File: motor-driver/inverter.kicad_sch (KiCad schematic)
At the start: 37 parts

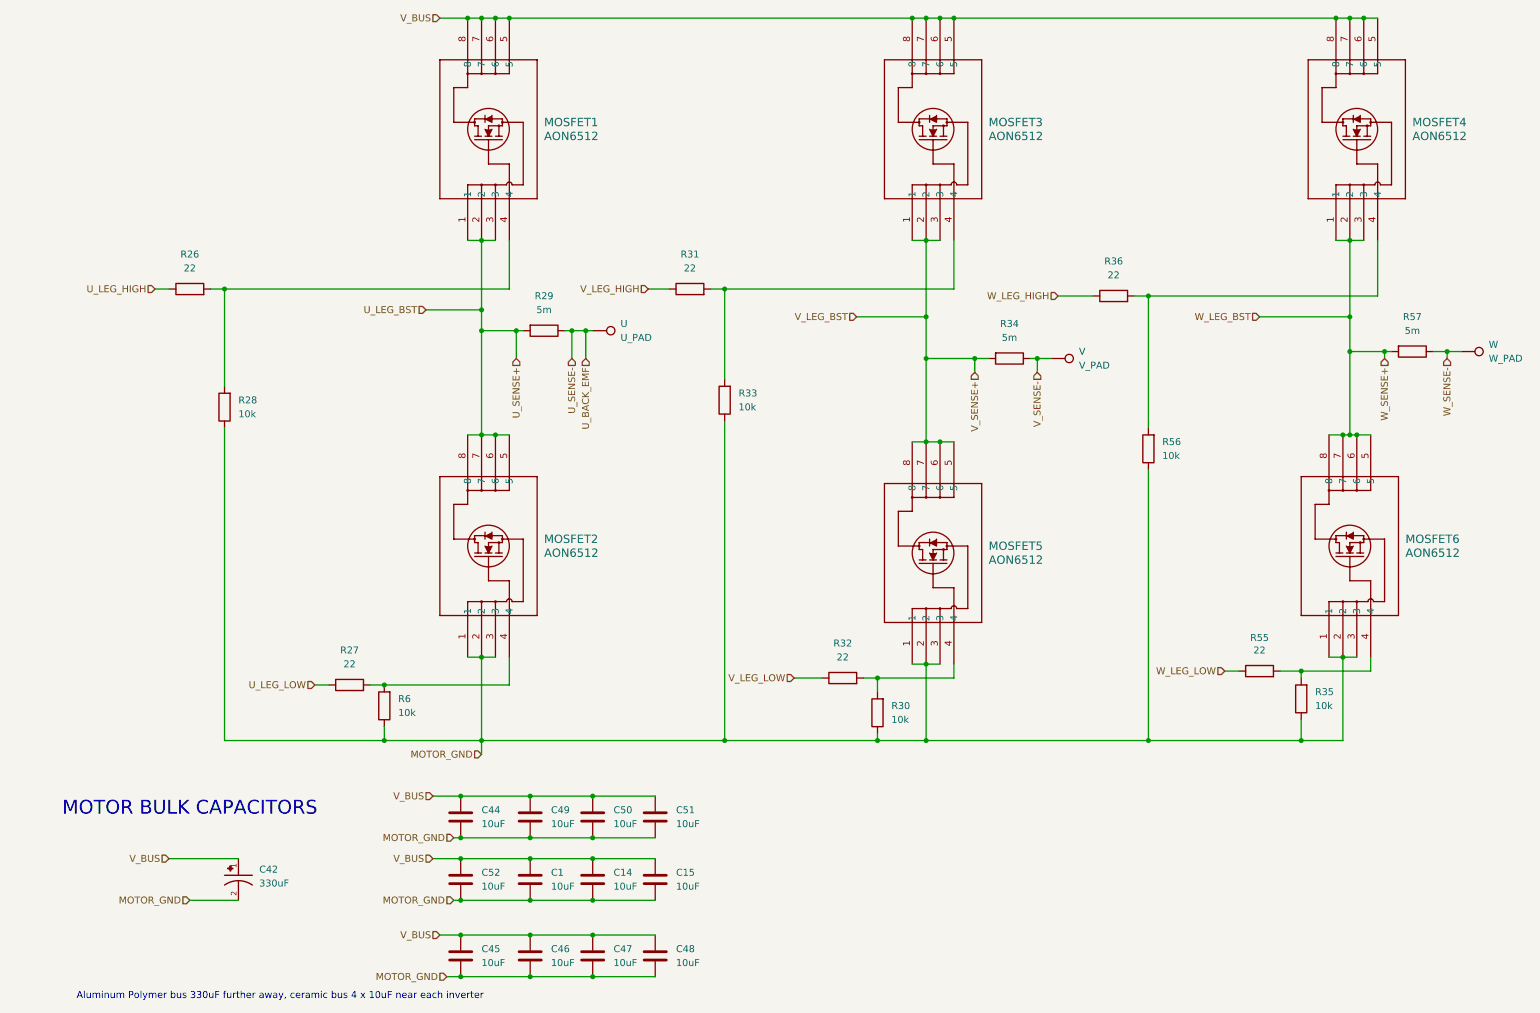
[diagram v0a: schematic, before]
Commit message: post revisions
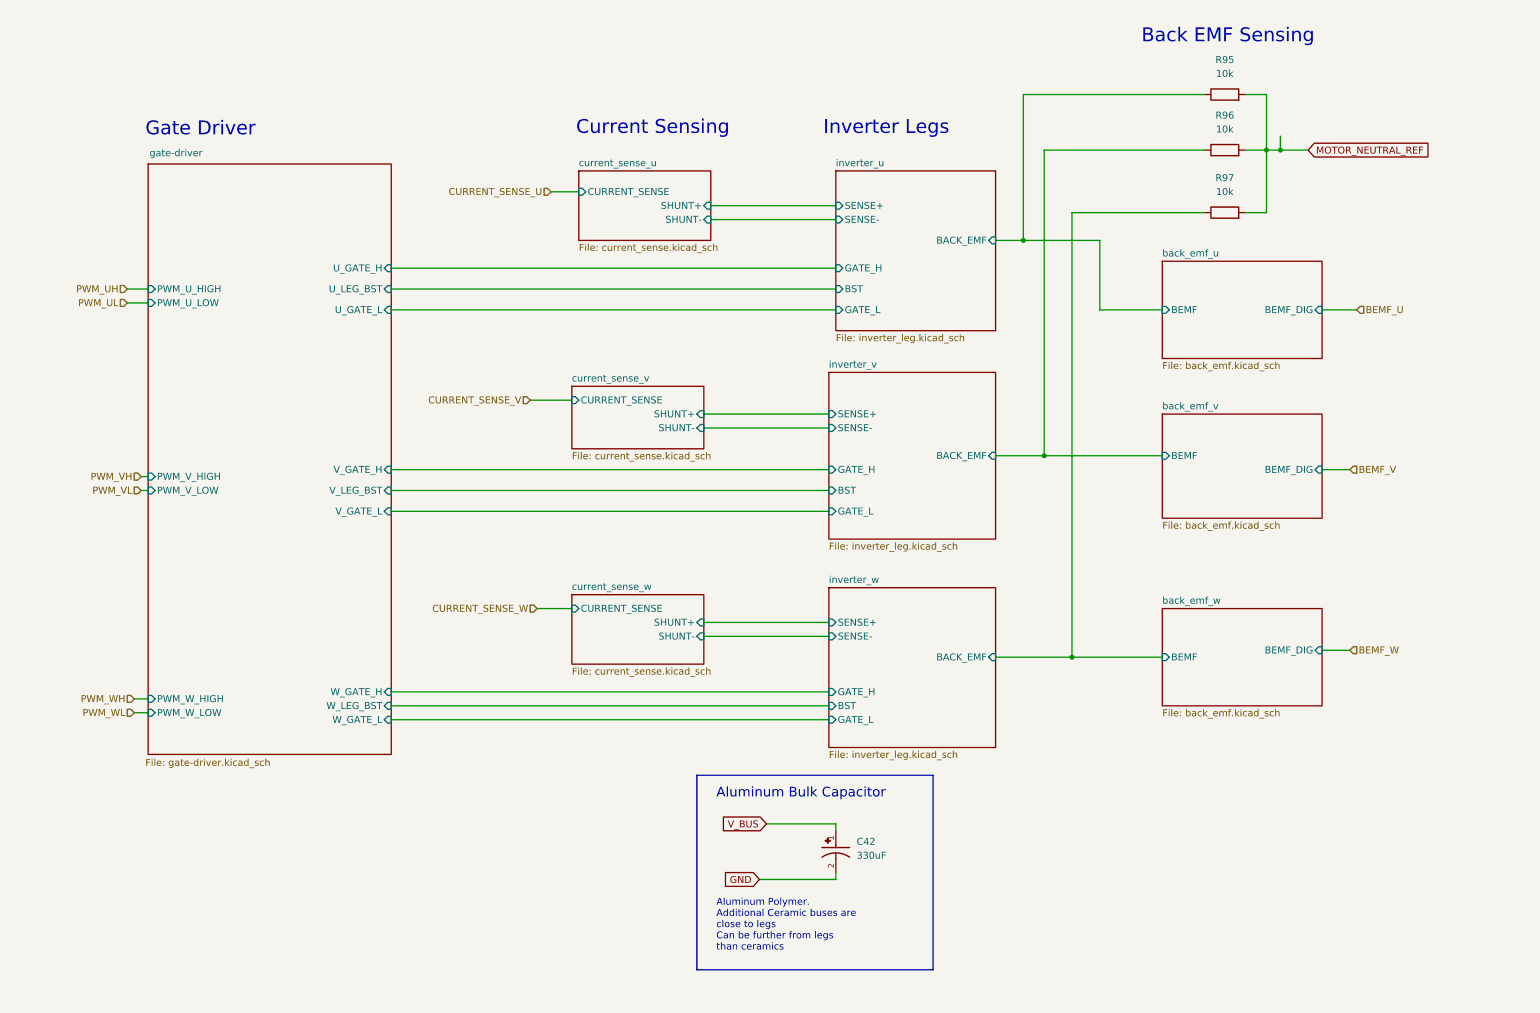
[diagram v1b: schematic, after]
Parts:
- removed C1, C14, C15, C44, C45, C46, C47, C48, C49, C50, C51, C52: 10uF, Capacitor_SMD:C_0603_1608Metric, symbol Device:C
- removed MOSFET1, MOSFET2, MOSFET3, MOSFET4, MOSFET5, MOSFET6: AON6512, AON6512:DFN5X6_8L_EP1_P_AOS, symbol AON6512:AON6512
- removed R26, R27, R31, R32, R36, R55: 22, Resistor_SMD:R_0603_1608Metric, symbol Device:R
- removed R28, R30, R33, R35, R56, R6: 10k, Resistor_SMD:R_0603_1608Metric, symbol Device:R
- removed R29, R34, R57: 5m, Resistor_SMD:R_2512_6332Metric, symbol Device:R
- removed U: U_PAD, symbol Connector:TestPoint
- removed V: V_PAD, symbol Connector:TestPoint
- removed W: W_PAD, symbol Connector:TestPoint
- added R95, R96, R97: 10k, Resistor_SMD:R_0603_1608Metric, symbol Device:R
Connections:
- net MOTOR_GND renamed GND
- new net MOTOR_NEUTRAL_REF: R95.2, R96.2, R97.2
- new net back_emf_u/BEMF: R95.1
- new net back_emf_v/BEMF: R96.1
- new net back_emf_w/BEMF: R97.1
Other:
- added sheet back_emf_u (back_emf.kicad_sch)
- added sheet back_emf_v (back_emf.kicad_sch)
- added sheet back_emf_w (back_emf.kicad_sch)
- added sheet current_sense_u (current_sense.kicad_sch)
- added sheet current_sense_v (current_sense.kicad_sch)
- added sheet current_sense_w (current_sense.kicad_sch)
- added sheet gate-driver (gate-driver.kicad_sch)
- added sheet inverter_u (inverter_leg.kicad_sch)
- added sheet inverter_v (inverter_leg.kicad_sch)
- added sheet inverter_w (inverter_leg.kicad_sch)
- note added: "Aluminum Bulk Capacitor"
- note added: "Aluminum Polymer. Additional Ceramic buses are close to legs Can be further from legs than ceramics"
- note added: "Back EMF Sensing"
- note added: "Current Sensing"
- note added: "Gate Driver"
- note added: "Inverter Legs"
- note removed: "Aluminum Polymer bus 330uF further away, ceramic bus 4 x 10uF near each inverter"
- note removed: "MOTOR BULK CAPACITORS"
- company: (none) -> Drone 
- moved on the sheet: C42
